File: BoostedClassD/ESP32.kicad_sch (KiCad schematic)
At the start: 10 parts, among them IC2 ESP32-WROOM-32UE-N8R2, IC3 RESET, IC4 BOOT

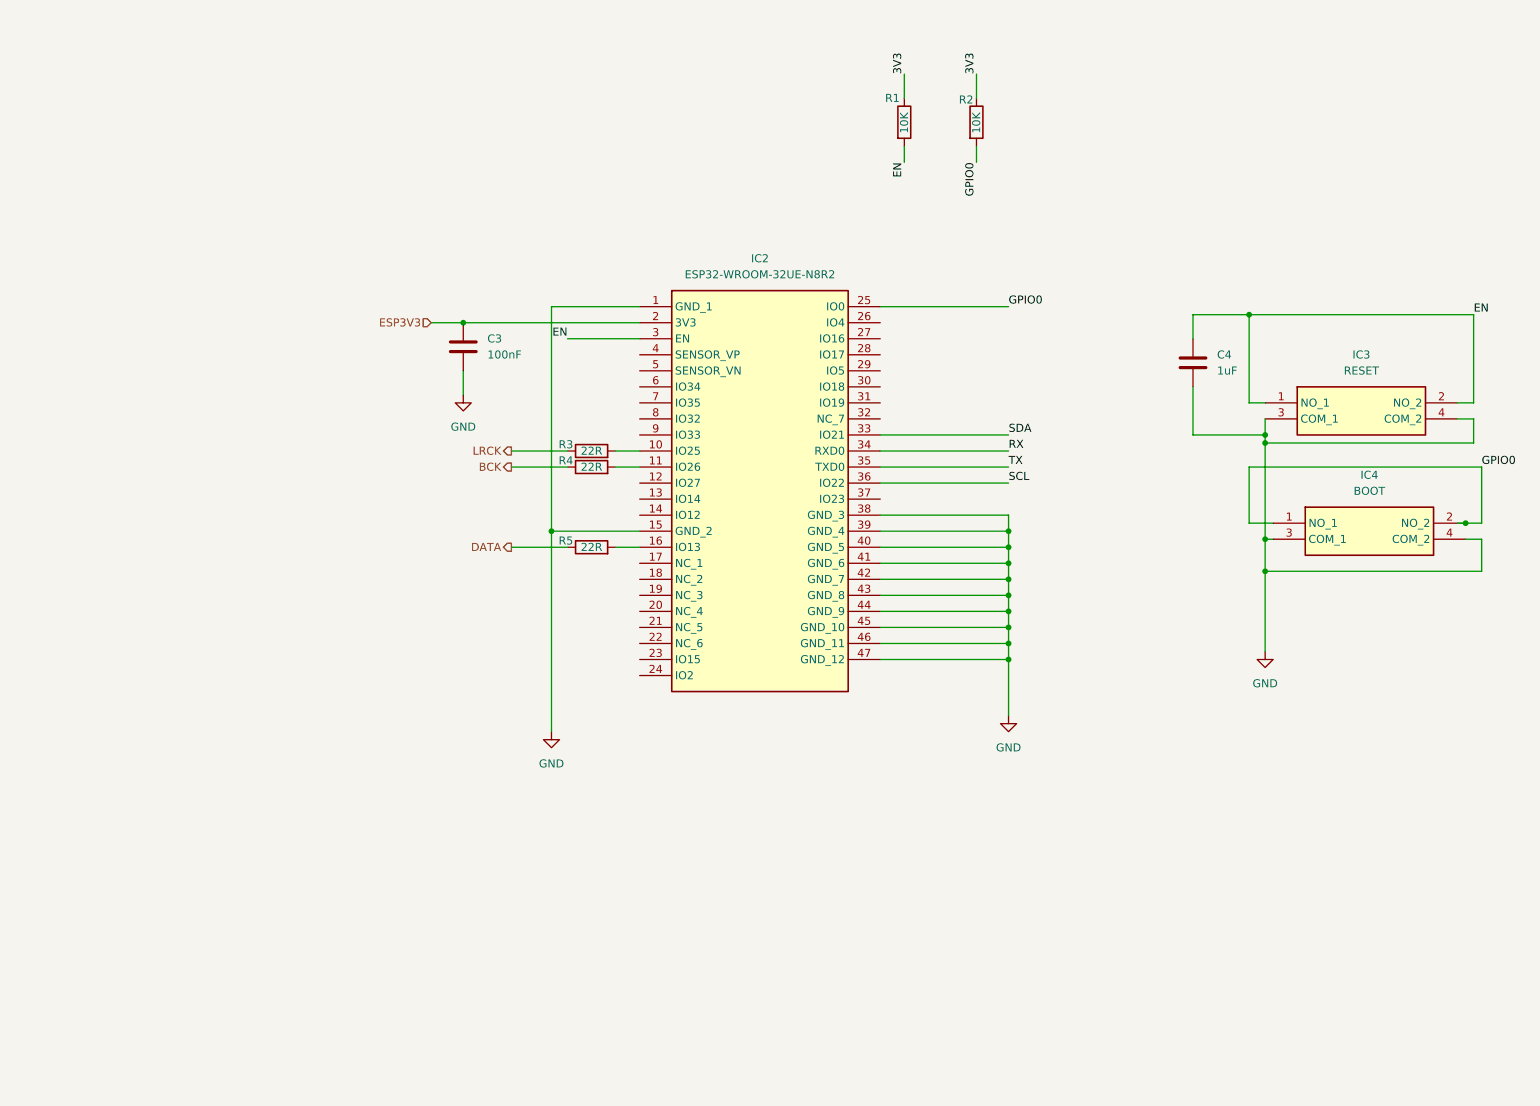
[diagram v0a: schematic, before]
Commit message: m0re
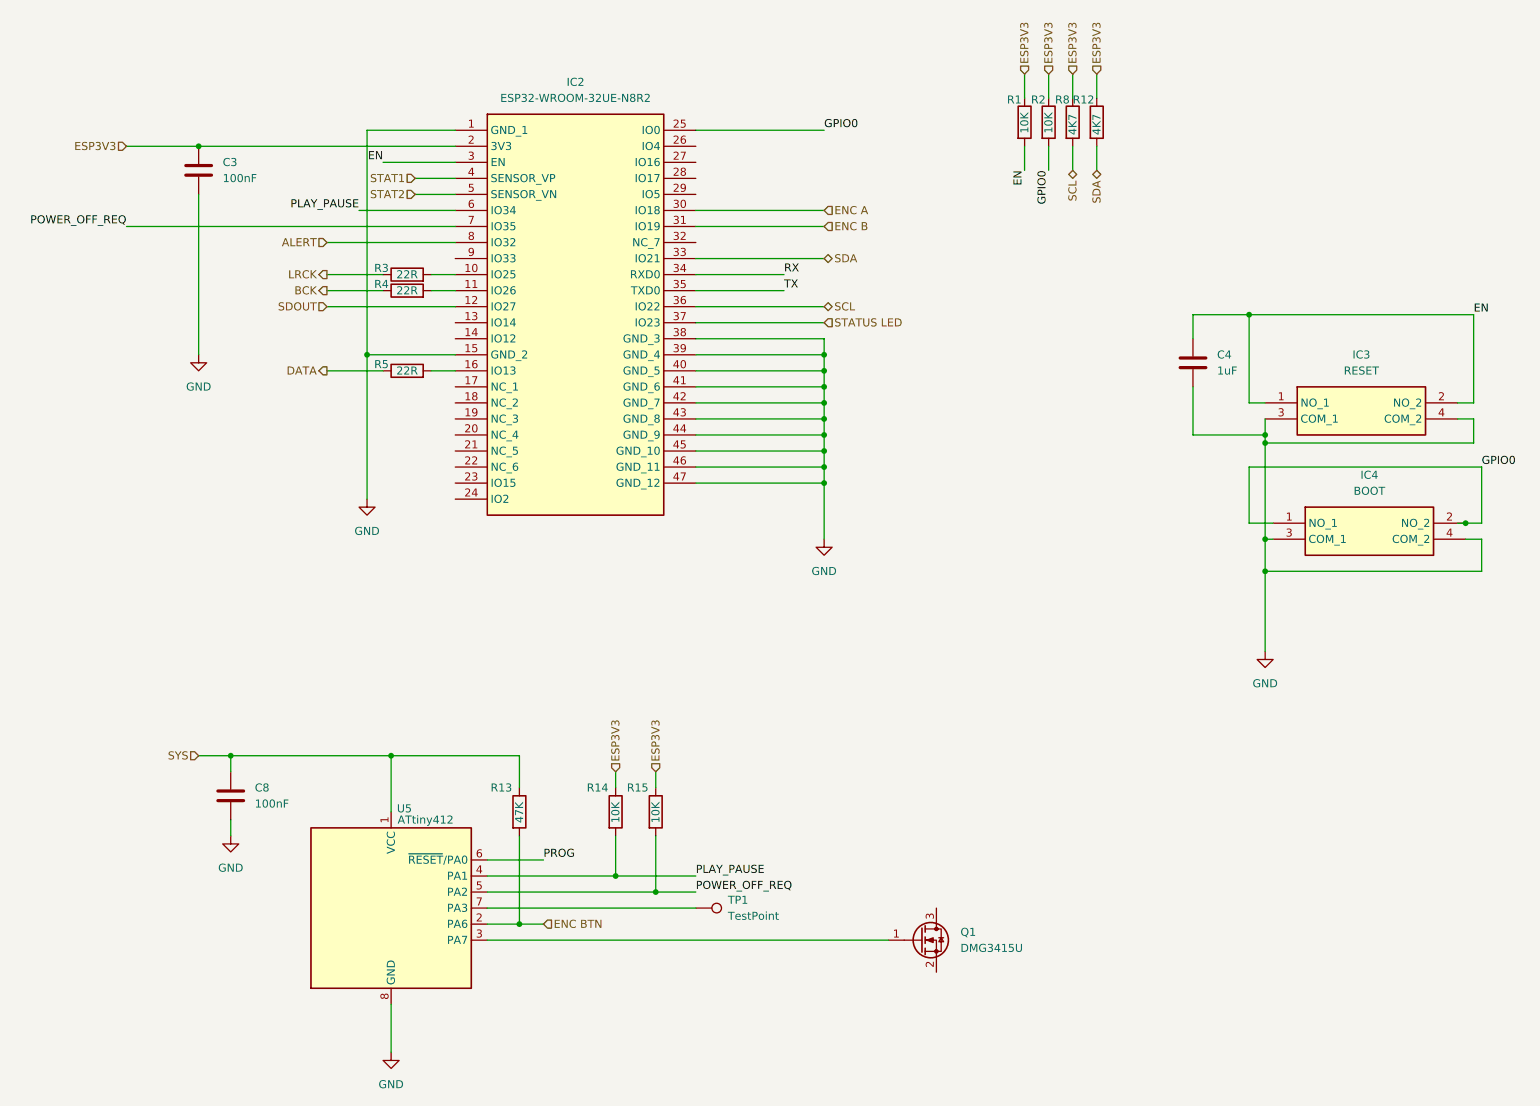
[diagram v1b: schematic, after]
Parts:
- added C8: 100nF, Capacitor_SMD:C_1206_3216Metric_Pad1.33x1.80mm_HandSolder, symbol Device:C
- added Q1: DMG3415U, Package_TO_SOT_SMD:SOT-23, symbol Transistor_FET:2N7002
- added R12, R8: 4K7, Resistor_SMD:R_0805_2012Metric_Pad1.20x1.40mm_HandSolder, symbol Device:R
- added R13: 47K, Resistor_SMD:R_0805_2012Metric_Pad1.20x1.40mm_HandSolder, symbol Device:R
- added R14, R15: 10K, Resistor_SMD:R_0805_2012Metric_Pad1.20x1.40mm_HandSolder, symbol Device:R
- added TP1: TestPoint, TestPoint:TestPoint_Pad_D2.0mm, symbol Connector:TestPoint
- added U5: ATtiny412, Package_SO:SOIC-8_3.9x4.9mm_P1.27mm, symbol MCU_Microchip_ATtiny:ATtiny412-SS
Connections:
- net 3V3 is gone; now on net ESP3V3: R1.1, R2.1
- net ESP3V3: now also R12.1, R14.1, R15.1, R8.1
- net GND: now also C8.2, U5.8 (GND)
- net SCL: now also R8.2
- net SDA: now also R12.2
- net SDOUT: now reaches IC2.12 (IO27)
- net ENC A: now reaches IC2.30 (IO18)
- net ENC B: now reaches IC2.31 (IO19)
- net STATUS LED: now reaches IC2.37 (IO23)
- net STAT1: now reaches IC2.4 (SENSOR_VP)
- net STAT2: now reaches IC2.5 (SENSOR_VN)
- net PLAY_PAUSE: now reaches IC2.6 (IO34)
- net PLAY_PAUSE: now also R14.2, U5.4 (PA1)
- net POWER_OFF_REQ: now reaches IC2.7 (IO35)
- net POWER_OFF_REQ: now also R15.2, U5.5 (PA2)
- net ALERT: now reaches IC2.8 (IO32)
- new net: TP1.1, U5.7 (PA3)
- new net: Q1.1 (G), U5.3 (PA7)
- new net ENC BTN: R13.2, U5.2 (PA6)
- new net PROG: U5.6 (~{RESET}/PA0)
- new net SYS: C8.1, R13.1, U5.1 (VCC)
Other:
- moved on the sheet: C3, IC2, R1, R2, R3, R4, R5
